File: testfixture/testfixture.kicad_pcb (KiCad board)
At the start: 2 copper layers, 21 x 30 mm, 4 parts, among them J101 Conn_Coaxial, J102 Conn_Coaxial, J103 632712000011

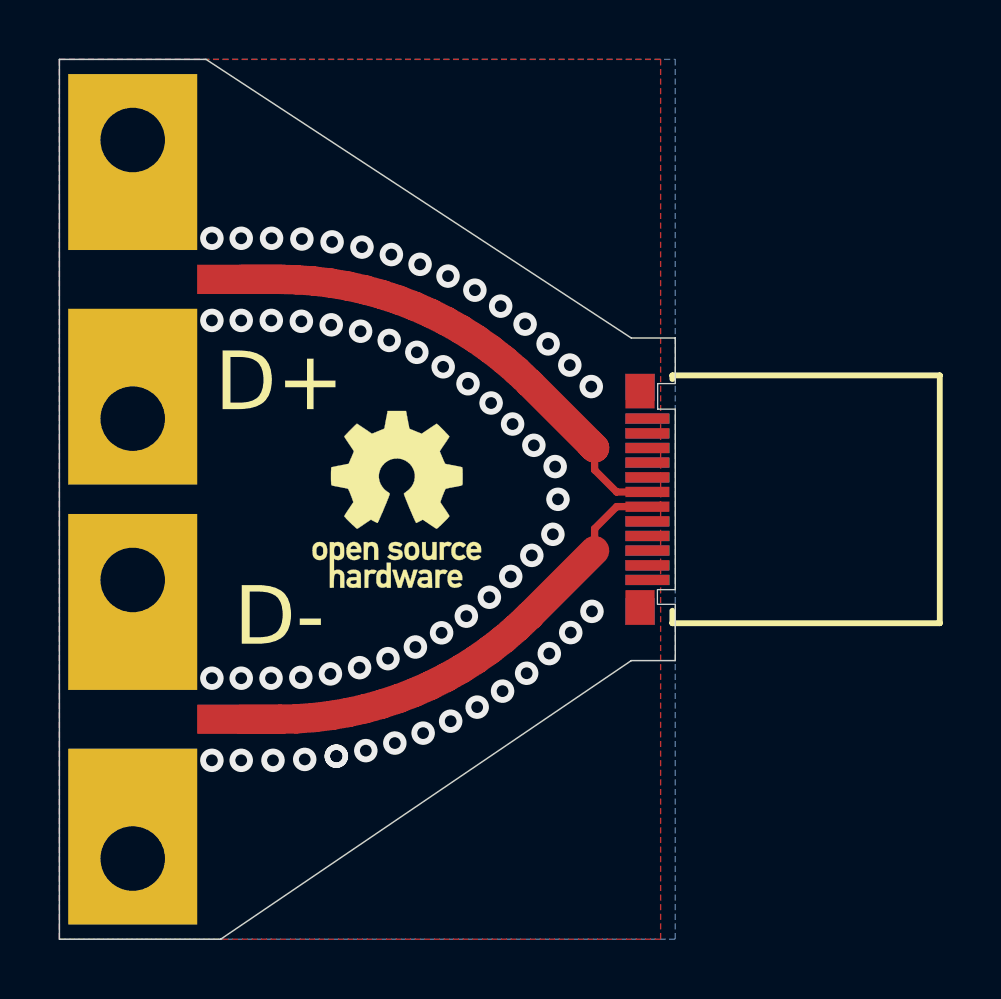
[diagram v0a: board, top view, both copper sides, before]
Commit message: Rev.B with Resistors and 45 Ohm matching
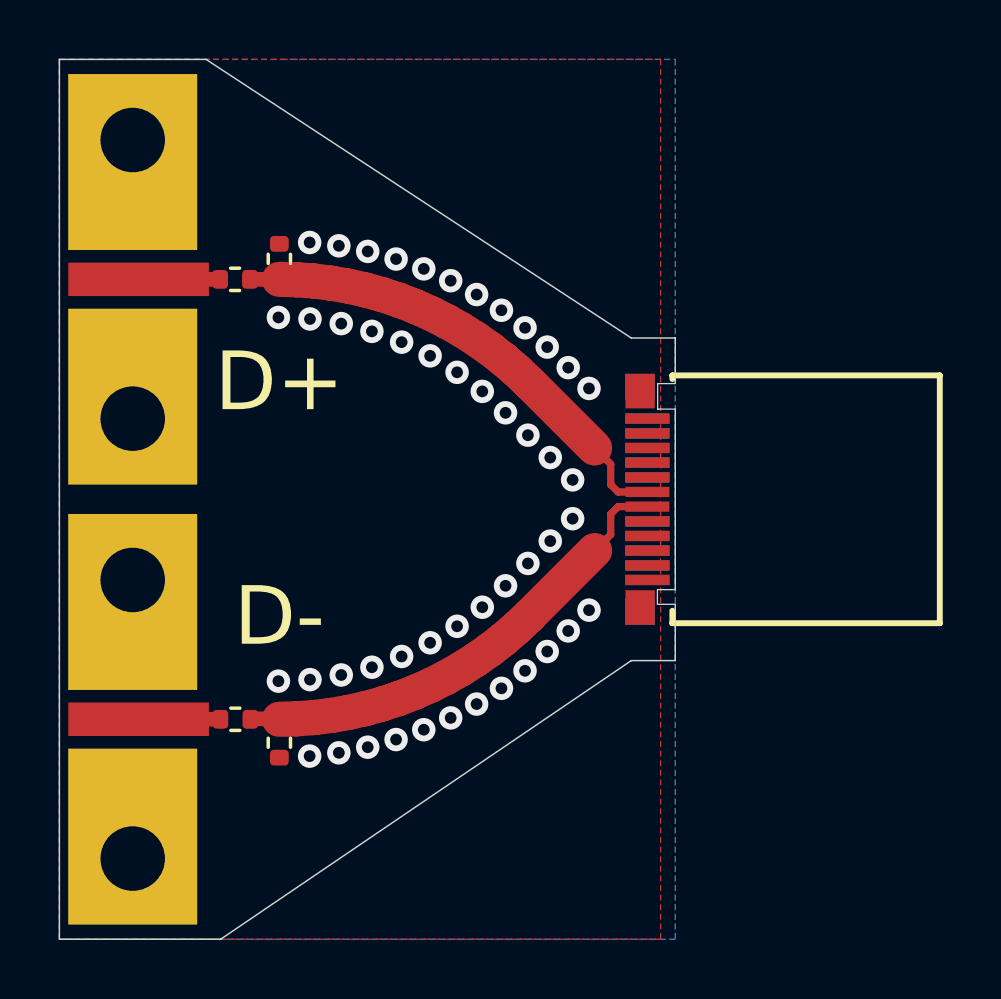
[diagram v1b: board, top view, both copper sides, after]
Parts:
- removed REF**: OSHW-Logo_5.7x6mm_SilkScreen, Symbol:OSHW-Logo_5.7x6mm_SilkScreen
- added R101: R, Resistor_SMD:R_0402_1005Metric, F.Cu at (136.0, 51.8)
- added R102: R, Resistor_SMD:R_0402_1005Metric, F.Cu at (136.0, 68.3)
- added R103: R, Resistor_SMD:R_0402_1005Metric, F.Cu at (134.5, 52.5)
- added R104: R, Resistor_SMD:R_0402_1005Metric, F.Cu at (134.5, 67.5)
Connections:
- J103 pad A6: Net-(J101-Pad1) -> Net-(J103-PadA6)
- J103 pad A7: Net-(J102-Pad1) -> Net-(J103-PadA7)
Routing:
- net Net-(J103-PadA7): track 0.00 -> 17.0 mm
- net Net-(J103-PadA6): track 0.00 -> 16.4 mm
- net Net-(J101-Pad1): track 16.9 -> 0.72 mm
- net Net-(J102-Pad1): track 16.7 -> 0.73 mm
- net GND: vias 60 -> 48
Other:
- net class 45ohm added: clearance 0.3, trace_width 1.2, via_dia 0.8, via_drill 0.4
- net class 50ohm removed
- board text added: "USB-C HS Testfixture Rev.B CC BY-SA 3.0 (c) 2022 Georg Ottinger"
- board text removed: "USB-C HS Testfixture CC BY-SA 3.0 (c) 2021 Georg Ottinger"
